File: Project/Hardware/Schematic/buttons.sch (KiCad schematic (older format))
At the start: 7 parts, among them U10 MomentSwitch, U11 MomentSwitch, U8 MomentSwitch, U9 MomentSwitch

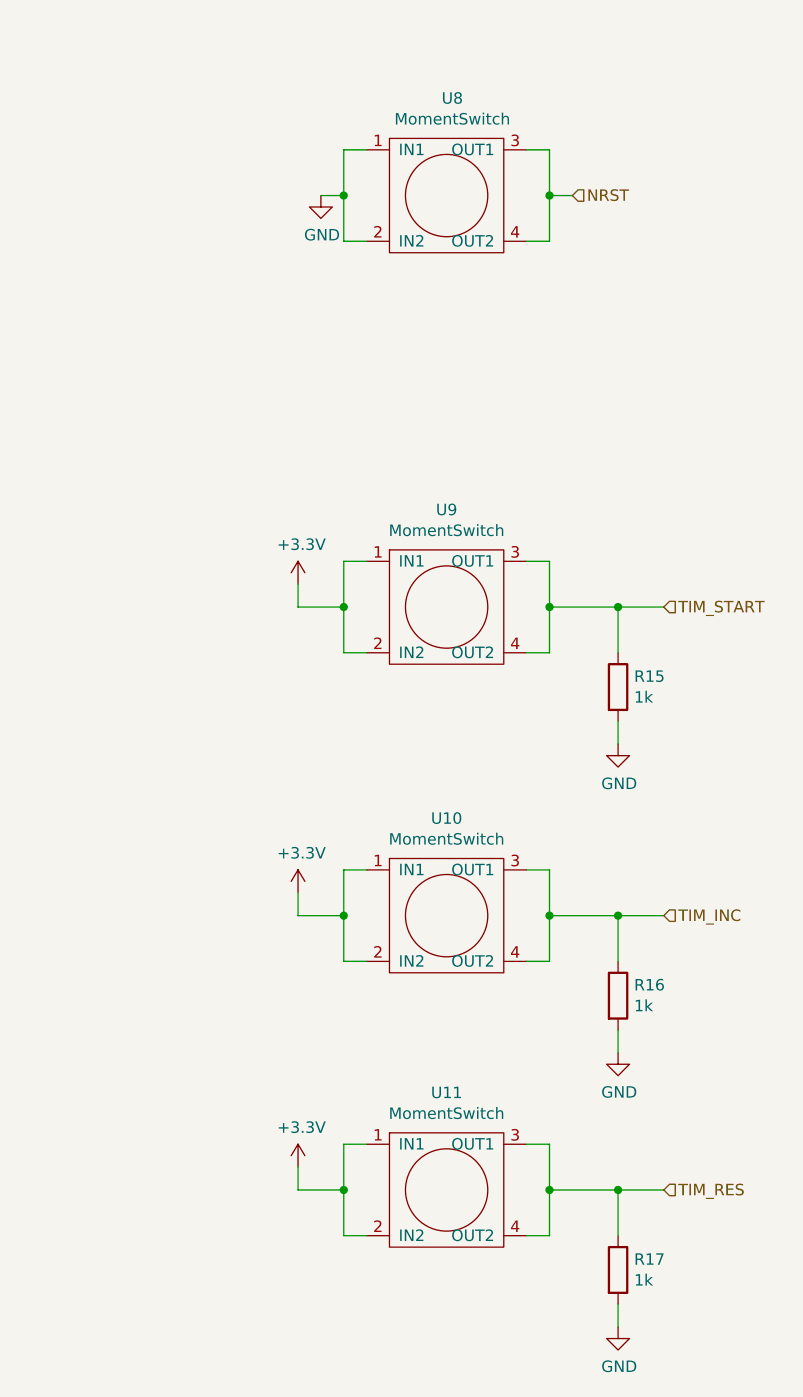
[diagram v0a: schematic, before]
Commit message: Intermediate...
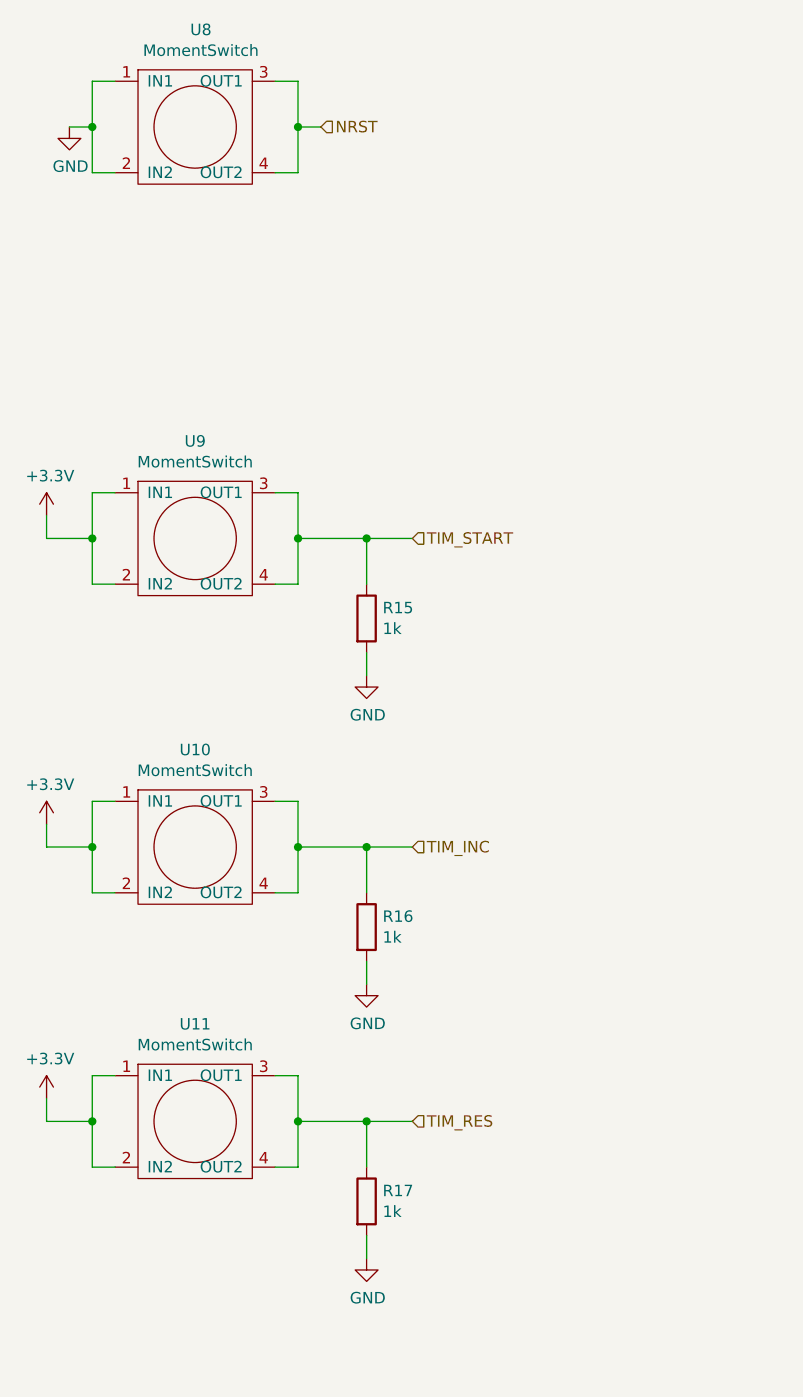
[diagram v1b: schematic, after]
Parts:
- R15, R16, R17: footprint (none) -> Resistor_SMD:R_0805_2012Metric_Pad1.15x1.40mm_HandSolder
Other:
- moved on the sheet: R15, R16, R17, U10, U11, U8, U9
